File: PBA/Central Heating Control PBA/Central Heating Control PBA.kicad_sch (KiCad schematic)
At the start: 158 parts

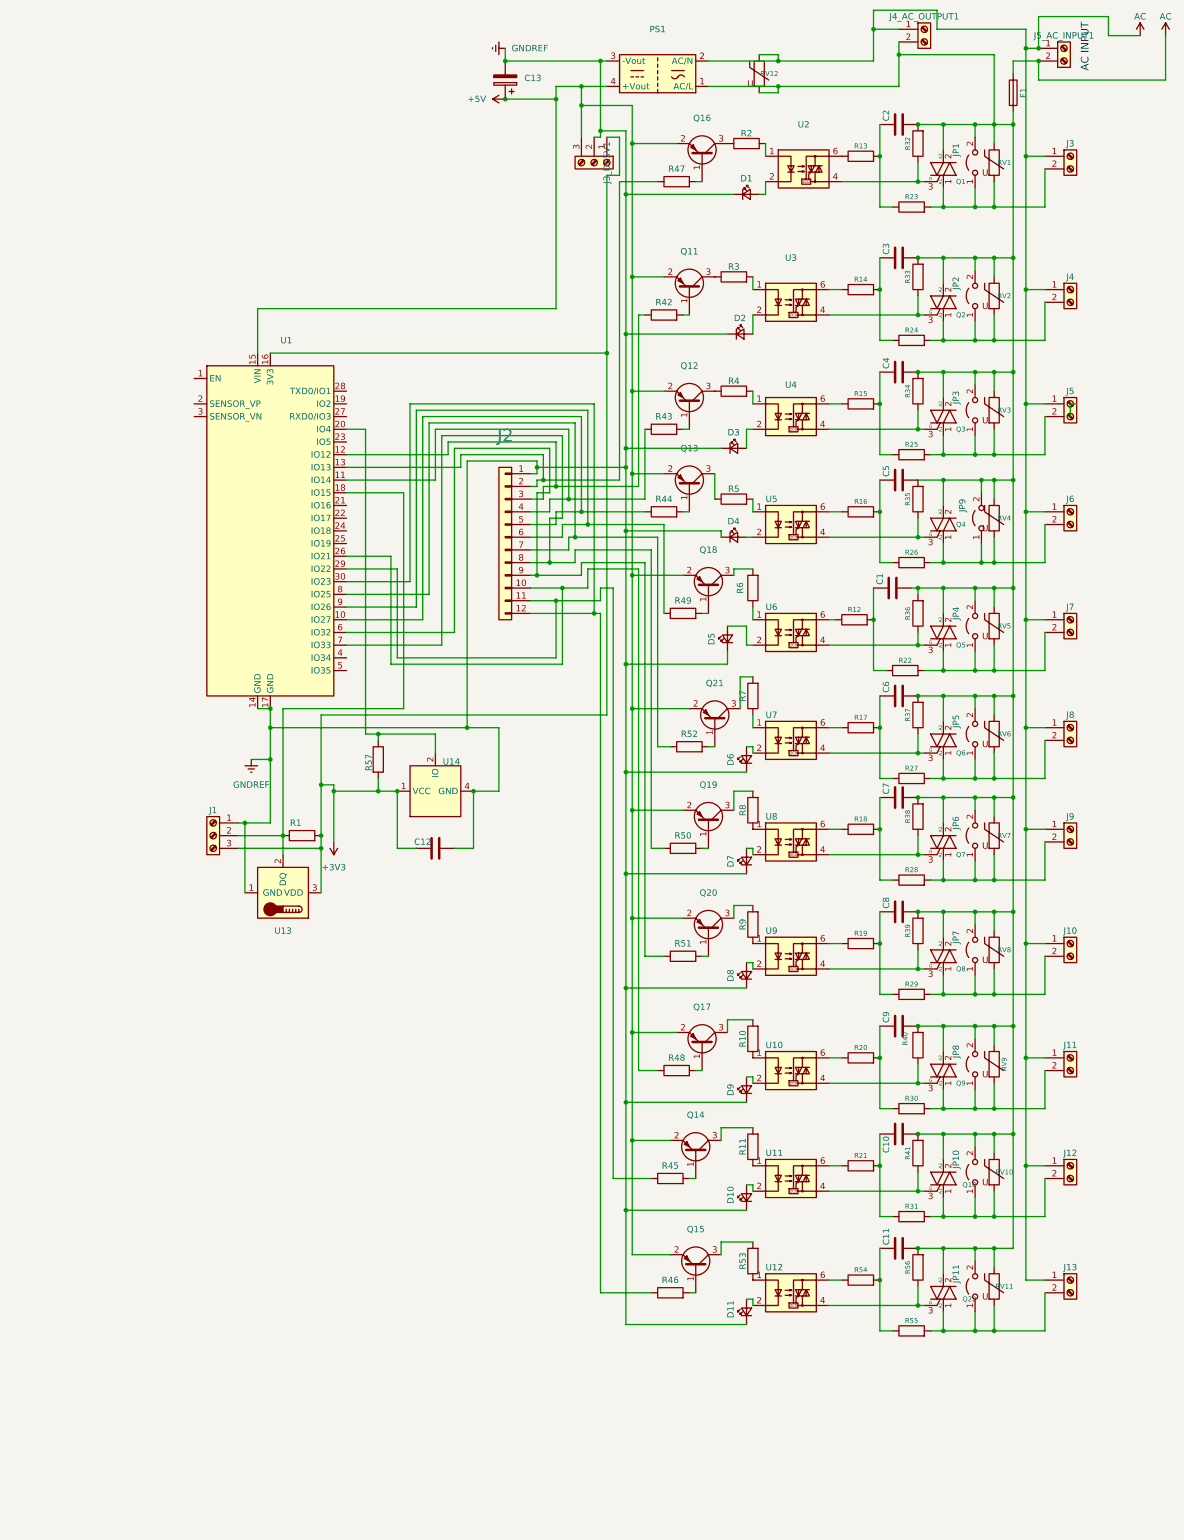
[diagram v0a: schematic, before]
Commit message: pba and code update
Signed-off-by: rgw <rgw@marm.pl>
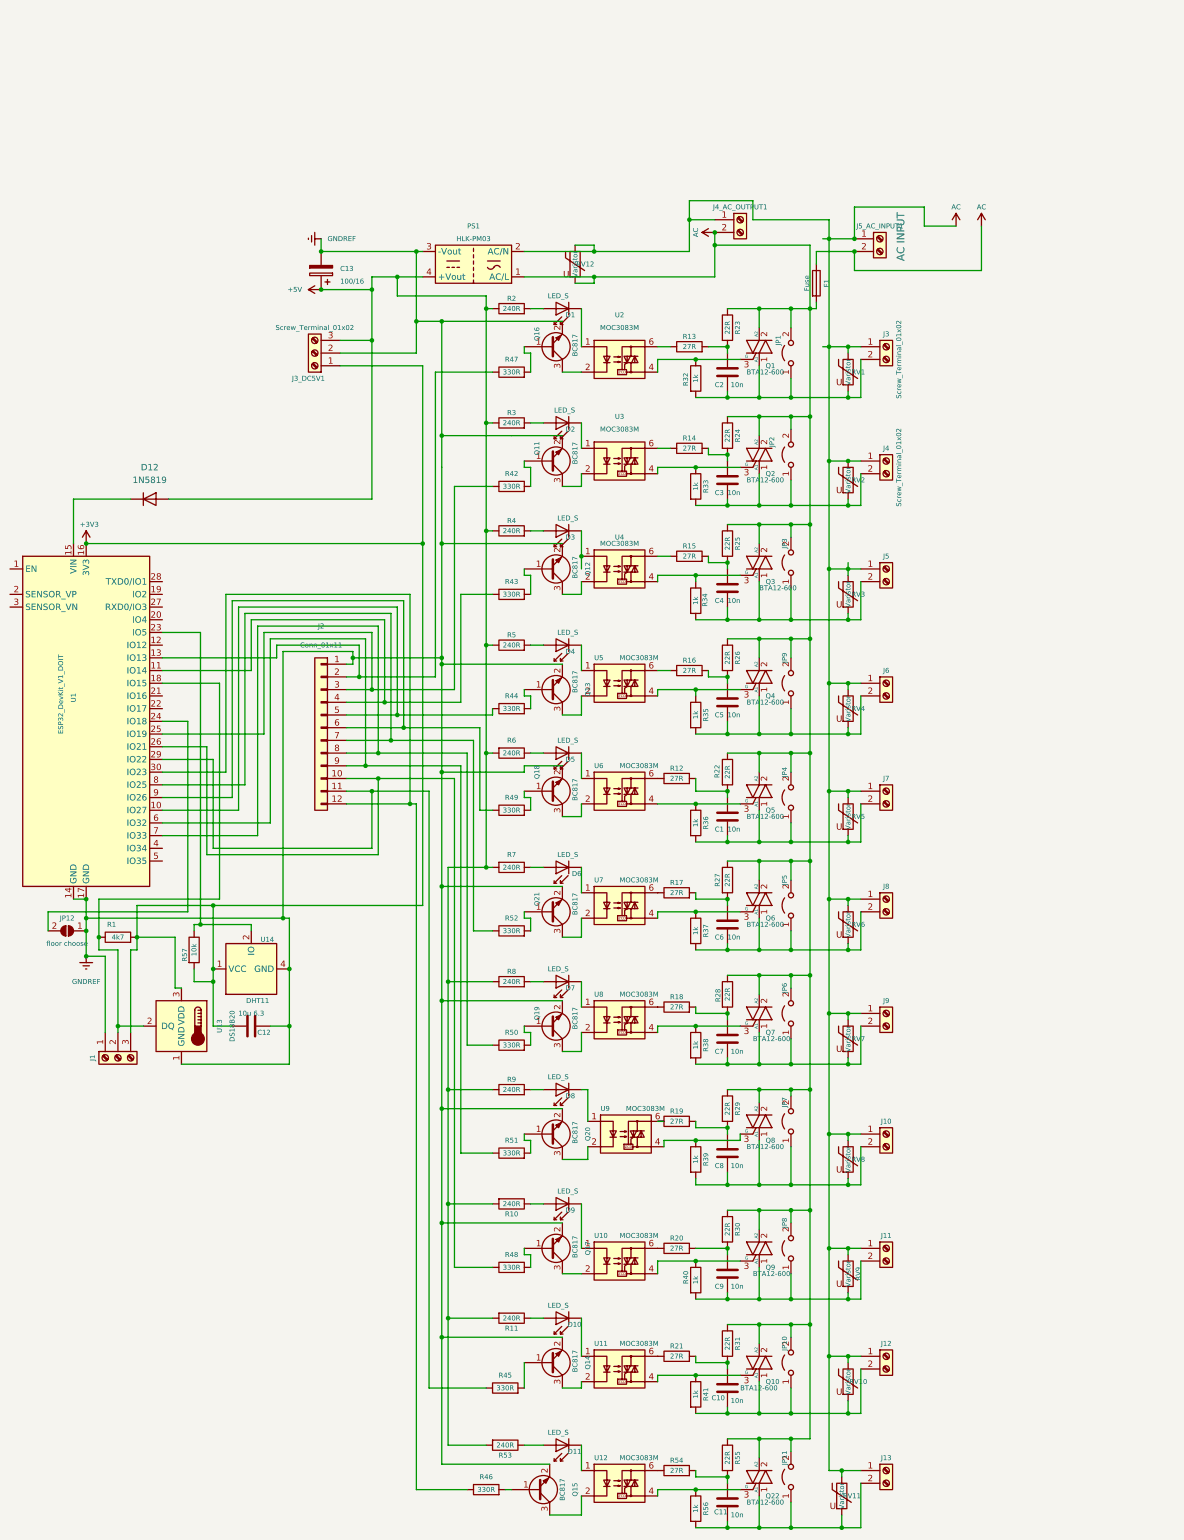
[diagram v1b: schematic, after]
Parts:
- added D12: 1N5819, Diode_SMD:D_SOD-123, symbol Diode:1N4148W
- added JP12: floor choose, Jumper:SolderJumper-2_P1.3mm_Open_TrianglePad1.0x1.5mm, symbol Jumper:SolderJumper_2_Open
- C1, C10, C11, C2, C3, C4, C5, C6, C7, C8, C9: value (none) -> 10n; footprint (none) -> Capacitor_THT:C_Rect_L19.0mm_W7.0mm_P15.00mm_MKS4
- C12: value (none) -> 10u 6.3; footprint (none) -> Capacitor_SMD:C_0805_2012Metric_Pad1.18x1.45mm_HandSolder
- C13: value (none) -> 100/16; footprint (none) -> Capacitor_SMD:CP_Elec_6.3x5.9; Spice_Model (none) -> 100n; Spice_Netlist_Enabled (none) -> Y; Spice_Primitive (none) -> C
- D1, D10, D11, D2, D3, D4, D5, D6, D7, D8, D9: value (none) -> LED_S; footprint (none) -> LED_THT:LED_Rectangular_W3.0mm_H2.0mm; symbol Untitled-rescue:LED_Small -> LED:IR204A
- F1: value (none) -> Fuse; footprint (none) -> Fuse:Fuseholder_Littelfuse_100_series_5x20mm
- J1: value (none) -> Screw_Terminal_01x03; footprint (none) -> TerminalBlock_MetzConnect:TerminalBlock_MetzConnect_Type086_RT03403HBLC_1x03_P3.81mm_Horizontal_hole-1.2
- J10, J11, J12, J13, J3, J4, J5, J6, J7, J8, J9: value (none) -> Screw_Terminal_01x02; footprint (none) -> TerminalBlock_MetzConnect:TerminalBlock_MetzConnect_Type171_RT13702HBWC_1x02_P7.50mm_Horizontal
- J2: value (none) -> Conn_01x11; footprint (none) -> Connector_PinHeader_2.54mm:PinHeader_1x12_P2.54mm_Vertical
- J3_DC5V1: value (none) -> Screw_Terminal_01x02; footprint (none) -> TerminalBlock_MetzConnect:TerminalBlock_MetzConnect_Type073_RT02603HBLU_1x03_P5.08mm_Horizontal
- J4_AC_OUTPUT1, J5_AC_INPUT1: value (none) -> Screw_Terminal_01x02; footprint (none) -> TerminalBlock_MetzConnect:TerminalBlock_MetzConnect_Type101_RT01602HBWC_1x02_P5.08mm_Horizontal
- JP1, JP10, JP11, JP2, JP3, JP4, JP5, JP6, JP7, JP8, JP9: value (none) -> Jumper_2_Open; footprint (none) -> Connector_PinSocket_2.54mm:PinSocket_1x02_P2.54mm_Vertical
- PS1: value (none) -> HLK-PM03; footprint (none) -> Converter_ACDC:Converter_ACDC_HiLink_HLK-PMxx; Spice_Model (none) -> dc 5; Spice_Netlist_Enabled (none) -> Y; Spice_Primitive (none) -> V
- Q1, Q10, Q2, Q22, Q3, Q4, Q5, Q6, Q7, Q8, Q9: value (none) -> BTA12-600; footprint (none) -> Package_TO_SOT_THT:TO-220-3_Vertical
- Q11, Q12, Q13, Q14, Q15, Q17, Q18, Q19, Q20, Q21: value (none) -> BC817; footprint (none) -> Package_TO_SOT_SMD:SOT-23; symbol Transistor_BJT:BC857 -> Transistor_BJT:BC817
- Q16: value (none) -> BC817; footprint (none) -> Package_TO_SOT_SMD:SOT-23; symbol Transistor_BJT:BC857 -> Transistor_BJT:BC817; Spice_Model (none) -> BC858; Spice_Netlist_Enabled (none) -> Y; Spice_Primitive (none) -> Q
- R1: value (none) -> 4k7; footprint (none) -> Resistor_SMD:R_0805_2012Metric_Pad1.20x1.40mm_HandSolder
- R10, R11, R2, R3, R4, R5, R53, R6, R7, R8, R9: value (none) -> 240R; footprint (none) -> Resistor_SMD:R_0805_2012Metric_Pad1.20x1.40mm_HandSolder
- R12, R13, R14, R15, R16, R17, R18, R19, R20, R21, R54: value (none) -> 27R; footprint (none) -> Resistor_THT:R_Axial_DIN0207_L6.3mm_D2.5mm_P2.54mm_Vertical
- R22, R23, R24, R25, R26, R27, R28, R29, R30, R31, R55: value (none) -> 22R; footprint (none) -> Resistor_THT:R_Axial_DIN0207_L6.3mm_D2.5mm_P2.54mm_Vertical
- R32, R33, R34, R35, R36, R37, R38, R39, R40, R41, R56: value (none) -> 1k; footprint (none) -> Resistor_THT:R_Axial_DIN0207_L6.3mm_D2.5mm_P2.54mm_Vertical
- R42, R43, R44, R45, R46, R47, R48, R49, R50, R51, R52: value (none) -> 330R; footprint (none) -> Resistor_SMD:R_0805_2012Metric_Pad1.20x1.40mm_HandSolder
- R57: value (none) -> 10k; footprint (none) -> Resistor_SMD:R_0805_2012Metric_Pad1.20x1.40mm_HandSolder
- RV1, RV10, RV11, RV12, RV2, RV3, RV4, RV5, RV6, RV7, RV8, RV9: value (none) -> Varistor; footprint (none) -> Varistor:RV_Disc_D9mm_W3.3mm_P5mm-hole0.9
- U1: value (none) -> ESP32_DevKit_V1_DOIT; footprint (none) -> Espressif:esp32_devkit_v1_doit
- U10, U11, U12, U2, U3, U4, U5, U6, U7, U8, U9: value (none) -> MOC3083M; footprint (none) -> Package_DIP:DIP-6_W7.62mm_LongPads_MOC3803
- U13: value (none) -> DS18B20; footprint (none) -> Package_TO_SOT_THT:TO-92_Inline_W4.0mm_Horizontal_FlatSideDown
- U14: value (none) -> DHT11; footprint (none) -> Sensor:Aosong_DHT11_5.5x12.0_P2.54mm
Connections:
- net +3V3: now also C12.2; no longer C12.1
- net +5V: now also R10.2, R11.2, R2.1, R3.1, R4.1, R5.1, R53.2, R6.2, R7.2, R8.1, R9.1, D12.2 (A); no longer Q11.2 (E), Q12.2 (E), Q13.2 (E), Q14.2 (E), Q15.2 (E), Q16.2 (E), Q17.2 (E), Q18.2 (E), Q19.2 (E), Q20.2 (E), Q21.2 (E), U1.15 (VIN)
- net GNDREF: now also C12.1, Q11.2 (E), Q12.2 (E), Q13.2 (E), Q14.2 (E), Q15.2 (E), Q16.2 (E), Q17.2 (E), Q18.2 (E), Q19.2 (E), Q20.2 (E), Q21.2 (E), JP12.1 (A); no longer C12.2, D1.1 (K), D10.1 (K), D11.1 (K), D2.1 (K), D3.1 (K), D4.1 (K), D5.1 (K), D6.1 (K), D7.1 (K), D8.1 (K), D9.1 (K)
- net LINE: now also F1.2, J4_AC_OUTPUT1.2 (Pin_2), JP1.2 (B), JP10.2 (B), JP11.2 (B), JP2.2 (B), JP3.2 (B), JP4.2 (B), JP5.2 (B), JP6.2 (B), JP7.2 (B), JP8.2 (B), JP9.2 (B), PS1.1 (AC/L), Q1.2 (A2), Q10.2 (A2), Q2.2 (A2), Q22.2 (A2), Q3.2 (A2), Q4.2 (A2), Q5.2 (A2), Q6.2 (A2), Q7.2 (A2), Q8.2 (A2), Q9.2 (A2), R22.1, R23.1, R24.1, R25.1, R26.1, R27.1, R28.1, R29.1, R30.1, R31.1, R55.1, RV12.2
- net NEUT: now also RV1.1, RV10.1, RV11.1, RV2.1, RV3.1, RV4.1, RV5.1, RV6.1, RV7.1, RV8.1, RV9.1
- net at U2.1: now also D1.1 (K); no longer R2.2
- net at U2.2: now also Q16.3 (C); no longer D1.2 (A)
- net at J3.2 (Pin_2), JP1.1 (A), Q1.1 (A1)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: now also C2.2, R32.2; no longer R23.2
- net at J2.3 (Pin_3), R42.1: now also U1.25 (IO19); no longer U1.12 (IO12)
- net at C2.1, R13.2: now also R23.2; no longer R23.1
- net at U3.1: now also D2.1 (K); no longer R3.2
- net at U3.2: now also Q11.3 (C); no longer D2.2 (A)
- net at J4.2 (Pin_2), JP2.1 (A), Q2.1 (A1)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: now also C3.2, R33.2; no longer R24.2
- net at C3.1, R14.2: now also R24.2; no longer R24.1
- net at U4.1: now also D3.1 (K); no longer R4.2
- net at U4.2: now also Q12.3 (C); no longer D3.2 (A)
- net at J5.2 (Pin_2), JP3.1 (A), Q3.1 (A1)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: now also C4.2, R34.2; no longer R25.2
- net at C4.1, R15.2: now also R25.2; no longer R25.1
- net at U5.1: now also D4.1 (K); no longer R5.2
- net at U5.2: now also Q13.3 (C); no longer D4.2 (A)
- net at J6.2 (Pin_2), JP9.1 (A), Q4.1 (A1)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: now also C5.2, R35.2; no longer R26.2
- net at C5.1, R16.2: now also R26.2; no longer R26.1
- net at U6.1: now also D5.1 (K); no longer R6.1
- net at U6.2: now also Q18.3 (C); no longer D5.2 (A)
- net at J7.2 (Pin_2), JP4.1 (A), Q5.1 (A1)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: now also C1.2, R36.2; no longer R22.2
- net at C1.1, R12.2: now also R22.2; no longer R22.1
- net at U7.1: now also D6.1 (K); no longer R7.1
- net at U7.2: now also Q21.3 (C); no longer D6.2 (A)
- net at J8.2 (Pin_2), JP5.1 (A), Q6.1 (A1)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: now also C6.2, R37.2; no longer R27.2
- net at C6.1, R17.2: now also R27.2; no longer R27.1
- net at U8.1: now also D7.1 (K); no longer R8.1
- net at U8.2: now also Q19.3 (C); no longer D7.2 (A)
- net at J9.2 (Pin_2), JP6.1 (A), Q7.1 (A1)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: now also C7.2, R38.2; no longer R28.2
- net at R8.2: now also D7.2 (A); no longer Q19.3 (C)
- net at C7.1, R18.2: now also R28.2; no longer R28.1
- net at U9.1: now also D8.1 (K); no longer R9.1
- net at U9.2: now also Q20.3 (C); no longer D8.2 (A)
- net at J10.2 (Pin_2), JP7.1 (A), Q8.1 (A1)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: now also C8.2, R39.2; no longer R29.2
- net at R9.2: now also D8.2 (A); no longer Q20.3 (C)
- net at C8.1, R19.2: now also R29.2; no longer R29.1
- net at U10.1: now also D9.1 (K); no longer R10.1
- net at U10.2: now also Q17.3 (C); no longer D9.2 (A)
- net at J11.2 (Pin_2), JP8.1 (A), Q9.1 (A1)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: now also C9.2, R40.2; no longer R30.2
- net at C9.1, R20.2: now also R30.2; no longer R30.1
- net at U11.1: now also D10.1 (K); no longer R11.1
- net at U11.2: now also Q14.3 (C); no longer D10.2 (A)
- net at J12.2 (Pin_2), JP10.1 (A), Q10.1 (A1)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: now also C10.2, R41.2; no longer R31.2
- net at C10.1, R21.2: now also R31.2; no longer R31.1
- net at J13.2 (Pin_2), JP11.1 (A), Q22.1 (A1)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: now also C11.2, R56.2; no longer R55.2
- net at R53.1: now also D11.2 (A); no longer U12.1
- net at Q15.3 (C): now also U12.2; no longer R53.2
- net at C11.1, R54.2: now also R55.2; no longer R55.1
- net at R57.1, U14.2 (IO): now also U1.23 (IO5); no longer U1.20 (IO4)
- net at U1.24 (IO18): now also JP12.2 (B)
- new net: D1.2 (A), R2.2
- new net: D2.2 (A), R3.2
- new net: D3.2 (A), R4.2
- new net: D4.2 (A), R5.2
- new net: D5.2 (A), R6.1
- new net: D6.2 (A), R7.1
- new net: D9.2 (A), R10.1
- new net: D10.2 (A), R11.1
- new net: D11.1 (K), U12.1
- new net: D12.1 (K), U1.15 (VIN)
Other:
- title: Modul wykonawczy CO 8termozaworow + pąpa CO podloga -> Modul wykonawczy CO 8termozaworow + pąpa CO +2zaw.4d?
- moved on the sheet: C1, C10, C11, C13, C2, C3, C4, C5, C6, C7, C8, C9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
